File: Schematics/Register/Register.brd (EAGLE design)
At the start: 132.1 x 84.8 mm, 42 parts

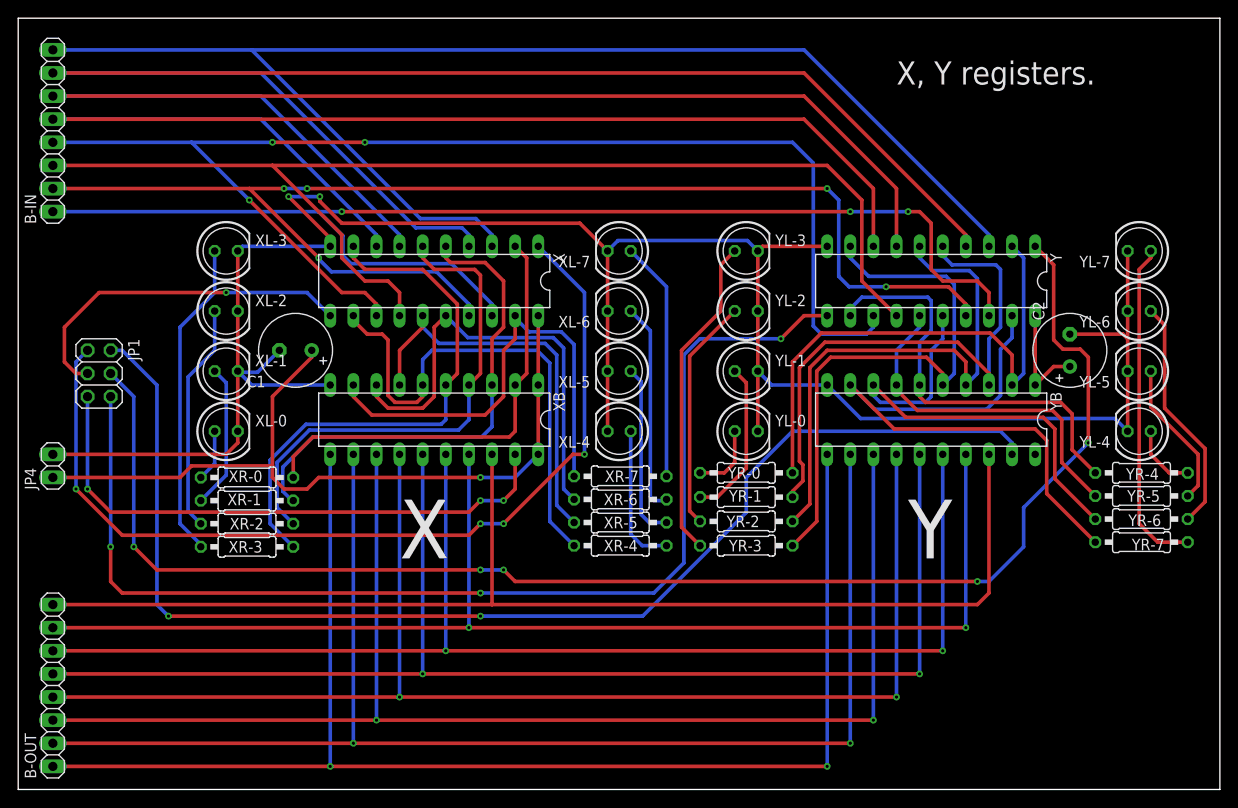
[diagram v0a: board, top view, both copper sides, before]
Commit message: Added register.
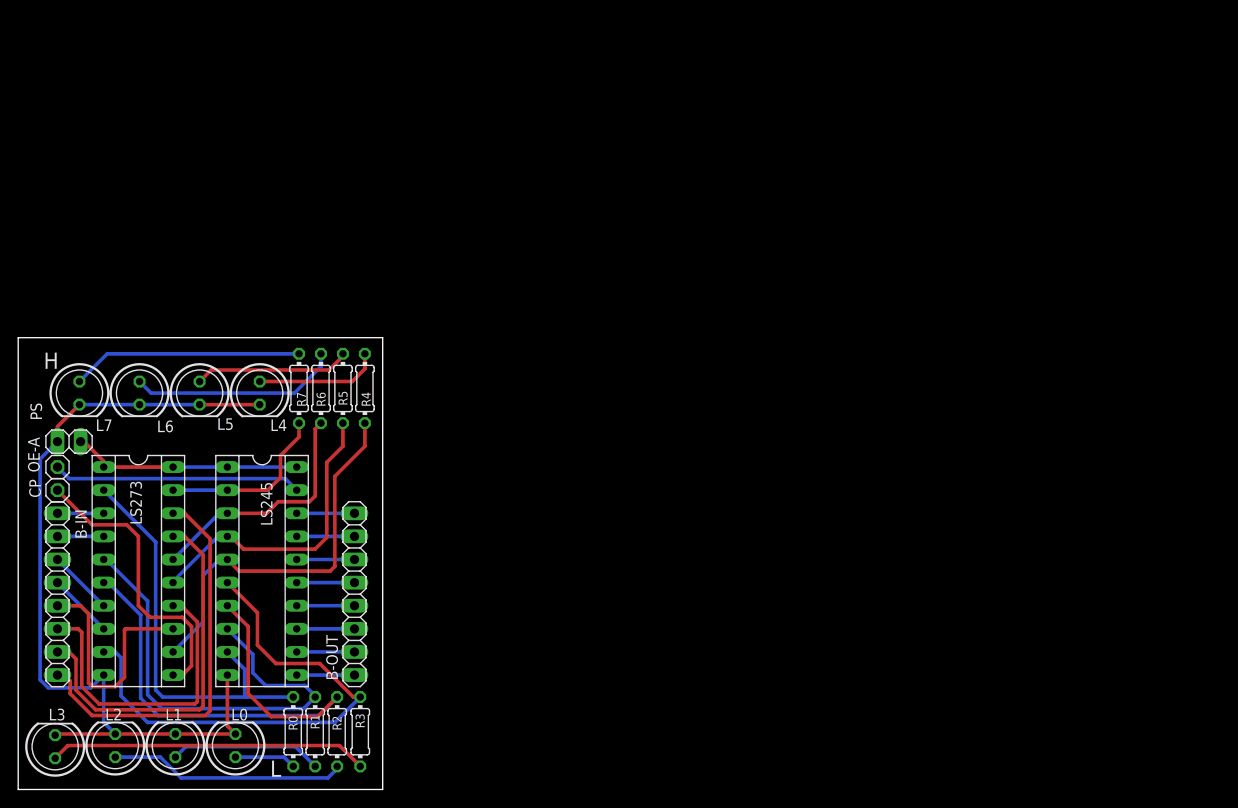
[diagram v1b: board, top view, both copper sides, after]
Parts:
- removed C1, C2: (no value), rcl:E3,5-8
- removed JP1: (no value), pinhead:2X03
- removed JP4: (no value), pinhead:1X02
- removed X, Y: 74273N, 74ttl-din:DIL20
- removed XB, YB: 74245N, 74ttl-din:DIL20
- removed XL-0, XL-1, XL-2, XL-3, XL-4, XL-5, XL-6, XL-7, YL-0, YL-1, YL-2, YL-3, YL-4, YL-5, YL-6, YL-7: (no value), led:LED5MM
- removed XR-0, XR-1, XR-2, XR-3, XR-4, XR-5, XR-6, XR-7, YR-0, YR-1, YR-2, YR-3, YR-4, YR-5, YR-6, YR-7: (no value), rcl:0207/10
- added CP, OE-A: (no value), pinhead:1X01
- added L0, L1, L2, L3, L4, L5, L6, L7: (no value), led:LED5MM
- added LS245, LS273: (no value), ic-package:SOCKET-20
- added PS: (no value), pinhead:1X02
- added R0, R1, R2, R3, R4, R5, R6, R7: (no value), rcl:0204/7
- moved B-IN 50.9 mm to (4.32, 21.5), turned to 270 degrees
- moved B-OUT 34.6 mm to (37.0, 21.5), turned to 270 degrees
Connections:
- removed net BI-0: B-IN.8, X.3, Y.3
- removed net BI-1: B-IN.7, X.4, Y.4
- removed net BI-2: B-IN.6, X.7, Y.7
- removed net BI-3: B-IN.5, X.8, Y.8
- removed net BI-4: B-IN.4, X.13, Y.13
- removed net BI-5: B-IN.3, X.14, Y.14
- removed net BI-6: B-IN.2, X.17, Y.17
- removed net BI-7: B-IN.1, X.18, Y.18
- removed net BO-0: B-OUT.8, XB.18, YB.18
- removed net BO-1: B-OUT.7, XB.17, YB.17
- removed net BO-2: B-OUT.6, XB.16, YB.16
- removed net BO-3: B-OUT.5, XB.15, YB.15
- removed net BO-4: B-OUT.4, XB.14, YB.14
- removed net BO-5: B-OUT.3, XB.13, YB.13
- removed net BO-6: B-OUT.2, XB.12, YB.12
- removed net BO-7: B-OUT.1, XB.11, YB.11
- removed net N$113: XL-1.A, XR-1.1
- removed net N$116: XL-2.A, XR-2.1
- removed net N$119: XL-3.A, XR-3.1
- removed net N$122: XL-4.A, XR-4.1
- removed net N$125: XL-5.A, XR-5.1
- removed net N$128: XL-6.A, XR-6.1
- removed net N$131: XL-7.A, XR-7.1
- removed net N$134: YL-0.A, YR-0.1
- removed net N$137: YL-1.A, YR-1.1
- removed net N$140: YL-2.A, YR-2.1
- removed net N$143: YL-3.A, YR-3.1
- removed net N$146: YL-4.A, YR-4.1
- removed net N$149: YL-5.A, YR-5.1
- removed net N$152: YL-6.A, YR-6.1
- removed net N$155: YL-7.A, YR-7.1
- removed net N$2: XL-0.A, XR-0.1
- removed net X-0: X.2, XB.2, XR-0.2
- removed net X-1: X.5, XB.3, XR-1.2
- removed net X-2: X.6, XB.4, XR-2.2
- removed net X-3: X.9, XB.5, XR-3.2
- removed net X-4: X.12, XB.6, XR-4.2
- removed net X-5: X.15, XB.7, XR-5.2
- removed net X-6: X.16, XB.8, XR-6.2
- removed net X-7: X.19, XB.9, XR-7.2
- removed net X-B: JP1.5, XB.19
- removed net X-CLR: JP1.1, X.1
- removed net X-CP: JP1.3, X.11
- removed net Y-0: Y.2, YB.2, YR-0.2
- removed net Y-1: Y.5, YB.3, YR-1.2
- removed net Y-2: Y.6, YB.4, YR-2.2
- removed net Y-3: Y.9, YB.5, YR-3.2
- removed net Y-4: Y.12, YB.6, YR-4.2
- removed net Y-5: Y.15, YB.7, YR-5.2
- removed net Y-6: Y.16, YB.8, YR-6.2
- removed net Y-7: Y.19, YB.9, YR-7.2
- removed net Y-B: JP1.2, YB.19
- removed net Y-CLR: JP1.4, Y.1
- removed net Y-CP: JP1.6, Y.11
- new net BO0: B-OUT.8, LS245.11
- new net BO1: B-OUT.7, LS245.12
- new net BO2: B-OUT.6, LS245.13
- new net BO3: B-OUT.5, LS245.14
- new net BO4: B-OUT.4, LS245.15
- new net BO5: B-OUT.3, LS245.16
- new net BO6: B-OUT.2, LS245.17
- new net BO7: B-OUT.1, LS245.18
- new net CP: CP.1, LS273.11
- new net D0: B-IN.1, LS273.3
- new net D1: B-IN.2, LS273.4
- new net D2: B-IN.3, LS273.7
- new net D3: B-IN.4, LS273.8
- new net D4: B-IN.5, LS273.13
- new net D5: B-IN.6, LS273.14
- new net D6: B-IN.7, LS273.17
- new net D7: B-IN.8, LS273.18
- new net N$1: L7.A, R7.1
- new net N$10: L1.A, R1.1
- new net N$11: L0.A, R0.1
- new net N$18: LS245.19, OE-A.1
- new net N$5: L6.A, R6.1
- new net N$6: L5.A, R5.1
- new net N$7: L4.A, R4.1
- new net N$8: L3.A, R3.1
- new net N$9: L2.A, R2.1
- new net Q0: LS245.9, LS273.2, R0.2
- new net Q1: LS245.8, LS273.5, R1.2
- new net Q2: LS245.7, LS273.6, R2.2
- new net Q3: LS245.6, LS273.9, R3.2
- new net Q4: LS245.5, LS273.12, R4.2
- new net Q5: LS245.4, LS273.15, R5.2
- new net Q6: LS245.3, LS273.16, R6.2
- new net Q7: LS245.2, LS273.19, R7.2
- net GND: now also L0.K, L1.K, L2.K, L3.K, L4.K, L5.K, L6.K, L7.K, LS245.10, LS273.10, PS.1; no longer C1.-, C2.-, JP4.2, X.10, XB.10, XL-0.K, XL-1.K, XL-2.K, XL-3.K, XL-4.K, XL-5.K, XL-6.K, XL-7.K, Y.10, YB.10, YL-0.K, YL-1.K, YL-2.K, YL-3.K, YL-4.K, YL-5.K, YL-6.K, YL-7.K
- net VCC: now also LS245.1, LS245.20, LS273.1, LS273.20, PS.2; no longer C1.+, C2.+, JP4.1, X.20, XB.1, XB.20, Y.20, YB.1, YB.20
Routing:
- net BI-1: track 163.3 -> 0.00 mm
- net Y-CLR: track 160.6 -> 0.00 mm, vias 5 -> 0
- net GND: track 248.4 -> 93.5 mm, vias 2 -> 0
- net BO-7: track 153.7 -> 0.00 mm, vias 2 -> 0
- net BO-6: track 151.1 -> 0.00 mm, vias 2 -> 0
- net BI-2: track 149.0 -> 0.00 mm
- net BI-0: track 148.7 -> 0.00 mm
- net BO-5: track 148.6 -> 0.00 mm, vias 2 -> 0
- net BO-4: track 146.0 -> 0.00 mm, vias 2 -> 0
- net BO-3: track 143.5 -> 0.00 mm, vias 2 -> 0
- net BI-6: track 142.5 -> 0.00 mm, vias 5 -> 0
- net BI-3: track 141.8 -> 0.00 mm
- net BO-2: track 141.0 -> 0.00 mm, vias 2 -> 0
- net BI-4: track 139.9 -> 0.00 mm, vias 3 -> 0
- net BO-1: track 138.4 -> 0.00 mm, vias 2 -> 0
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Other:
- board size 132.1 x 84.8 mm -> 40.1 x 49.6 mm
- board text added: "H"
- board text added: "L"
- board text removed: "X"
- board text removed: "X, Y registers."
- board text removed: "Y"
